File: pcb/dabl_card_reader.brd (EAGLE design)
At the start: 120 x 50 mm, 10 parts, among them U1 TEENSY_3.1_WITH_AUDIO

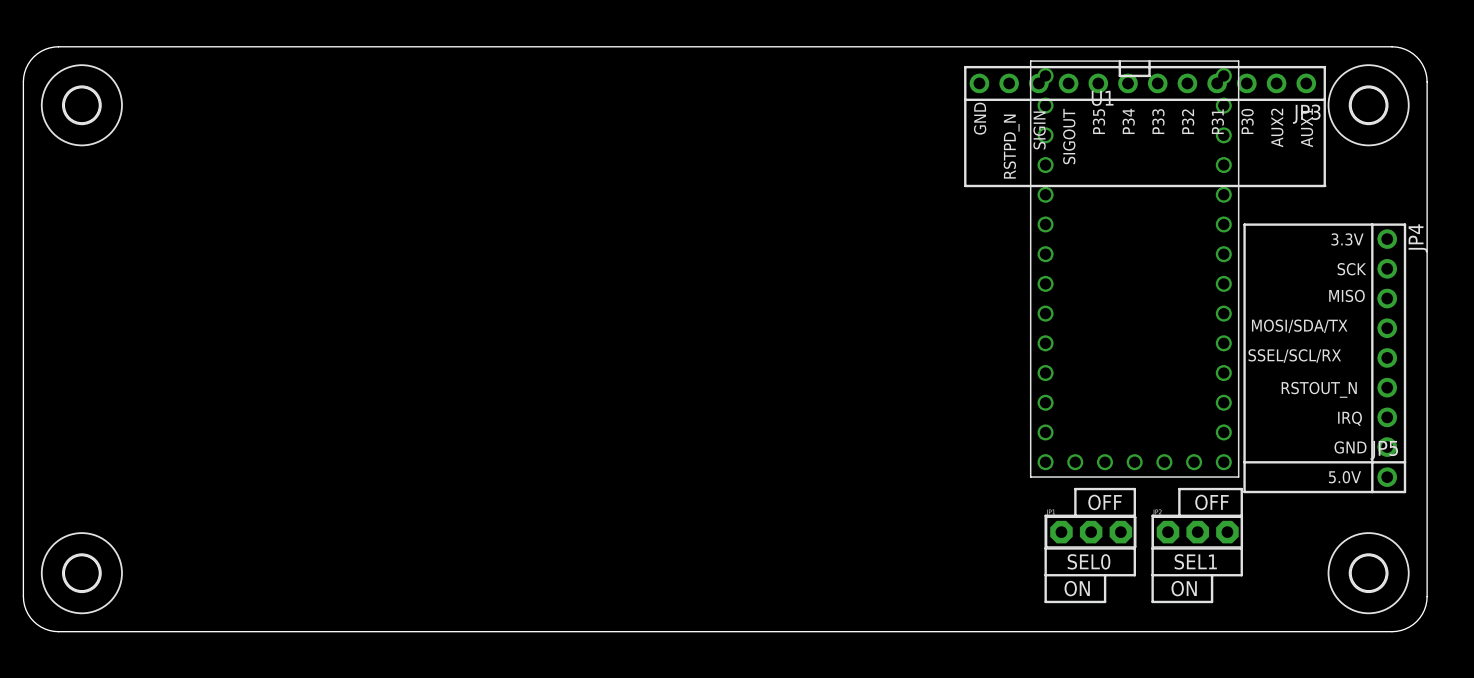
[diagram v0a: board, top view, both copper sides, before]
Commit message: full pcb for testing
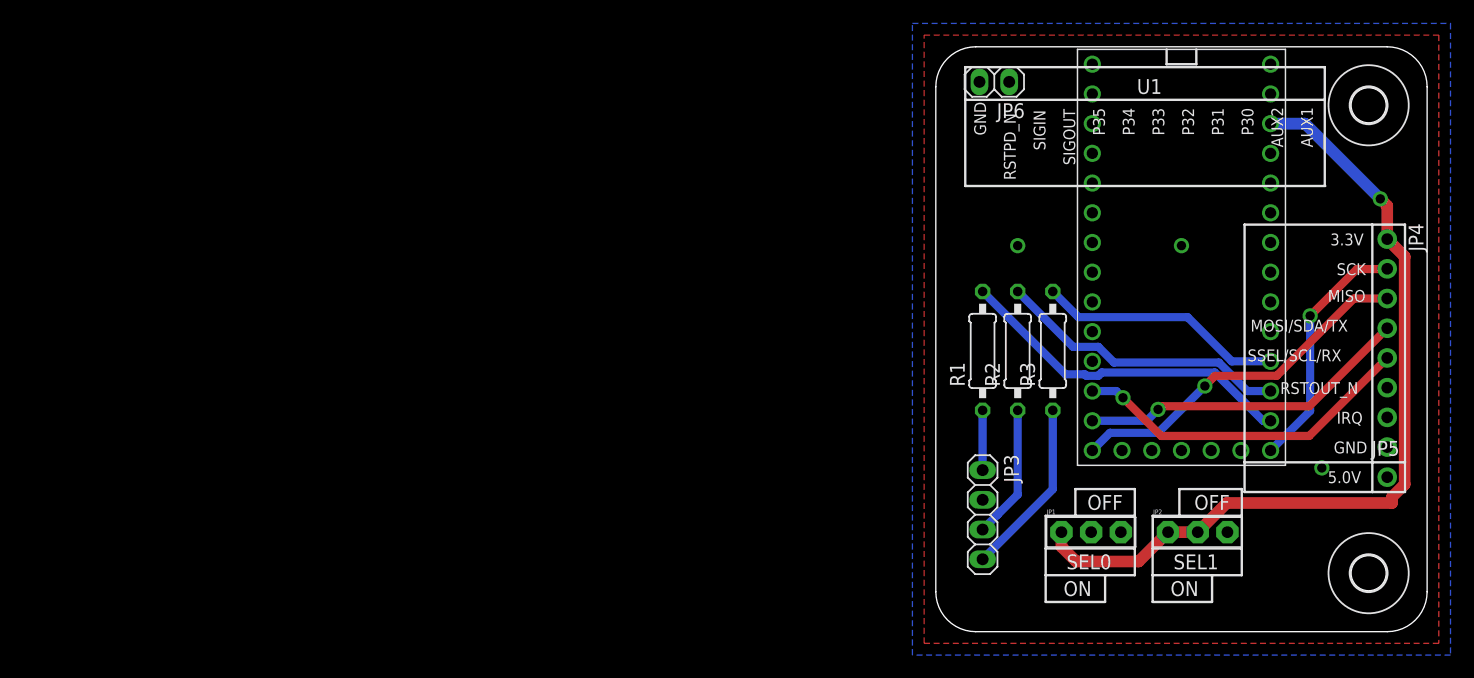
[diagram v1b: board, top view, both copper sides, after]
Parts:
- removed U$36, U$6: (no value), microbuilder:MOUNTINGHOLE_3.0
- added JP6: (no value), pinhead:1X02
- added R1, R2, R3: 220, resistor:0207/10
- JP3: device microbuilder:1X12_ROUND -> pinhead:1X04
- moved JP3 39.3 mm to (22.0, 10.0), turned to 270 degrees
- moved U1 4.12 mm to (39.0, 32.0)
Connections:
- removed net 3.3V: U1.3.3V, U1.3.3V1
- removed net MOSI/SDA/TX: JP4.4
- removed net NSS/SCL/RX: JP4.5
- removed net SEL0: JP1.2
- removed net SEL1: JP2.2
- new net CS: JP4.5, U1.10
- new net MOSI: JP4.4, U1.11
- new net N$1: JP3.4, R3.1
- new net N$10: R1.2, U1.14/A0
- new net N$2: JP3.3, R2.1
- new net N$5: JP3.1, R1.1
- new net N$8: R3.2, U1.16/A2
- new net N$9: R2.2, U1.15/A1
- net GND: now also JP1.2, JP3.2, JP6.2; no longer JP3.12
- net MISO: now also U1.12
- net SCK: now also U1.13
- net VDD: now also JP2.2, U1.3.3V, U1.3.3V1
- net VIN: no longer JP5.1
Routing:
- net VDD: track 0.00 -> 71.5 mm, vias 0 -> 1
- net MISO: track 0.00 -> 30.6 mm, vias 0 -> 1
- net CS: track 0.00 -> 29.6 mm, vias 0 -> 1
- net N$10: track 0.00 -> 29.4 mm
- net MOSI: track 0.00 -> 28.5 mm, vias 0 -> 1
- net N$9: track 0.00 -> 25.1 mm
- net SCK: track 0.00 -> 21.2 mm, vias 0 -> 1
- net N$8: track 0.00 -> 21.1 mm
- net N$1: track 0.00 -> 15.2 mm
- net N$2: track 0.00 -> 11.4 mm
- net N$5: track 0.00 -> 5.11 mm
- added copper zone on layer 1, net GND
- added copper zone on layer 16, net GND
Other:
- board size 120 x 50 mm -> 42 x 50 mm
